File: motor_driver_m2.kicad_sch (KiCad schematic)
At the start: 32 parts, among them J7 Conn_01x01_Pin, J8 Conn_01x01_Pin, J9 Conn_01x01_Pin, M2 DRV8320SRTVR, Q10 NP80N06D6, Q11 NP80N06D6, Q12 NP80N06D6, Q7 NP80N06D6, Q8 NP80N06D6, Q9 NP80N06D6

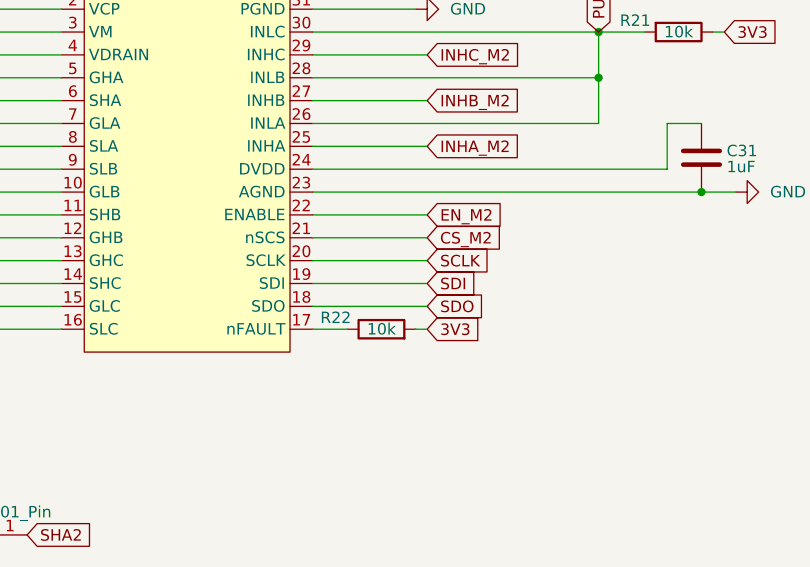
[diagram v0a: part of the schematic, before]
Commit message: ...
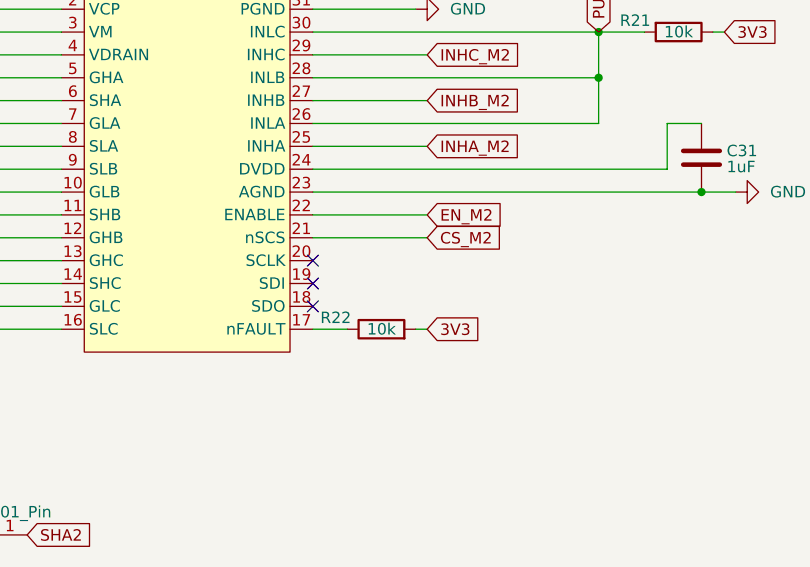
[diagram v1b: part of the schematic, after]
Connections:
- net SCLK: no longer names the net of M2.20 (SCLK)
- net SDI: no longer names the net of M2.19 (SDI)
- net SDO: no longer names the net of M2.18 (SDO)
- no-connect marks 0 -> 3
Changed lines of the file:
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@@
 		(color 0 0 0 0)
 	)
+	(no_connect
+		(at 92.71 80.01)
+	)
+	(no_connect
+		(at 92.71 77.47)
+	)
+	(no_connect
+		(at 92.71 74.93)
+	)
 	(wire
 		(pts
@@
 	(wire
 		(pts
-			(xy 105.41 74.93) (xy 92.71 74.93)
-		)
-		(stroke
-			(width 0)
-			(type default)
-		)
-	)
-	(wire
-		(pts
 			(xy 105.41 57.15) (xy 92.71 57.15)
 		)
@@
 	(wire
 		(pts
-			(xy 105.41 77.47) (xy 92.71 77.47)
-		)
-		(stroke
-			(width 0)
-			(type default)
-		)
-	)
-	(wire
-		(pts
 			(xy 77.47 161.29) (xy 77.47 162.56)
 		)
@@
 	(wire
 		(pts
-			(xy 92.71 80.01) (xy 105.41 80.01)
-		)
-		(stroke
-			(width 0)
-			(type default)
-		)
-	)
-	(wire
-		(pts
 			(xy 21.59 50.8) (xy 21.59 49.53)
 		)
@@
 		)
 	)
-	(global_label "SCLK"
-		(shape input)
-		(at 105.41 74.93 0)
-		(fields_autoplaced yes)
-		(effects
-			(font
-				(size 1.27 1.27)
-			)
-			(justify left)
-		)
-		(property "Intersheetrefs" "${INTERSHEET_REFS}"
-			(at 113.1728 74.93 0)
-			(effects
-				(font
-					(size 1.27 1.27)
-				)
-				(justify left)
-				(hide yes)
-			)
-		)
-	)
 	(global_label "B+"
 		(shape input)
@@
 		)
 	)
-	(global_label "SDO"
-		(shape input)
-		(at 105.41 80.01 0)
-		(fields_autoplaced yes)
-		(effects
-			(font
-				(size 1.27 1.27)
-			)
-			(justify left)
-		)
-		(property "Intersheetrefs" "${INTERSHEET_REFS}"
-			(at 112.2052 80.01 0)
-			(effects
-				(font
-					(size 1.27 1.27)
-				)
-				(justify left)
-				(hide yes)
-			)
-		)
-	)
 	(global_label "GLB2"
 		(shape input)
@@
 			(effects
 				(font
-					(size 1.27 1.27)
-				)
-				(justify left)
-				(hide yes)
-			)
-		)
-	)
-	(global_label "SDI"
-		(shape input)
-		(at 105.41 77.47 0)
-		(fields_autoplaced yes)
-		(effects
-			(font
-				(size 1.27 1.27)
-			)
-			(justify left)
-		)
-		(property "Intersheetrefs" "${INTERSHEET_REFS}"
-			(at 111.4795 77.47 0)
-			(effects
-				(font
